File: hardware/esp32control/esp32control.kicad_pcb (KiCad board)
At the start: 2 copper layers, 67.6 x 85.9 mm, 76 parts, among them J1 Conn_02x10_Odd_Even, Q1 BSS138, Q2 BSS138, Q3 BSS138, Q4 BSS138, Q5 BSS138, Q6 BSS138, Q7 MMBT3904, Q8 MMBT3904, SW1 Boot, SW2 Reset, U1 ESP32-WROOM, U10 LTV-354T, U11 HUT4, U12 LM1117-3.3, U2 AQY212, U3 AQY212, U4 LM2675M-5, U5 LTV-354T, U6 AQY212, U7 AQY212, U8 LTV-354T, U9 LTV-354T

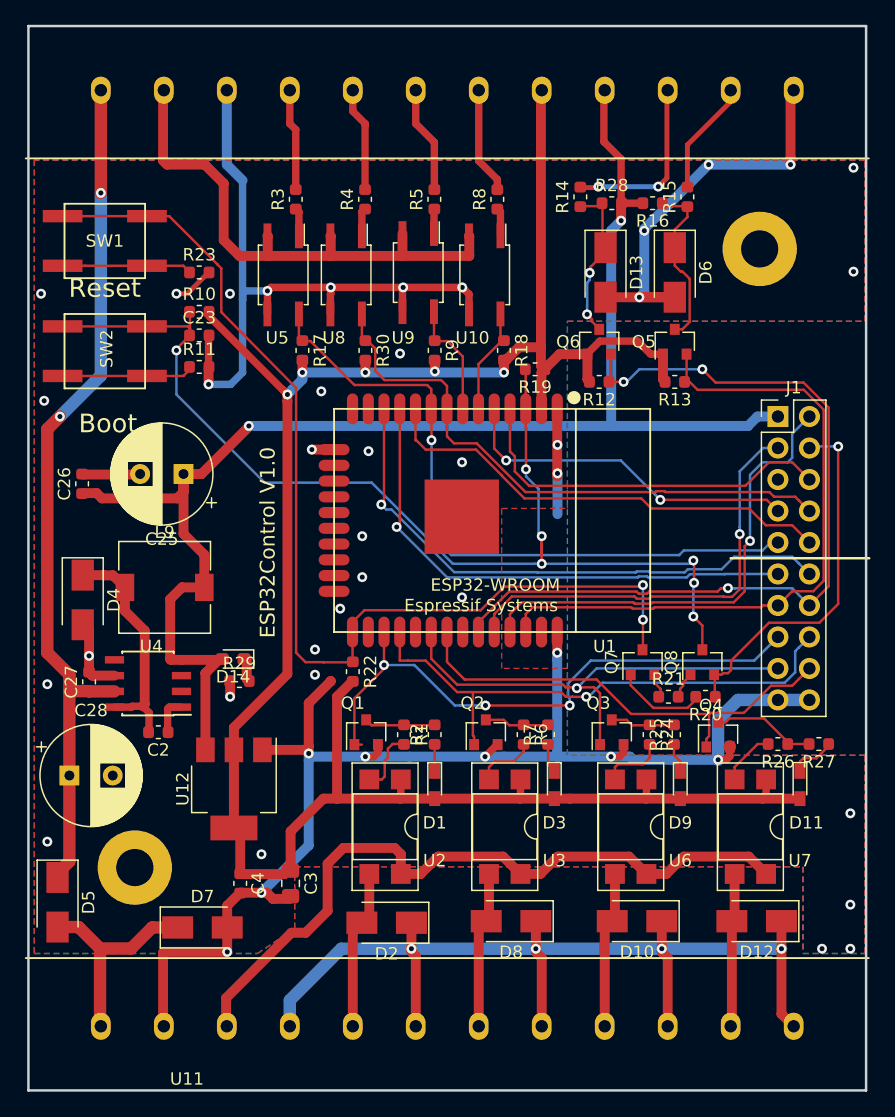
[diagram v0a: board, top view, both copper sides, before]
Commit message: silk update, fab files regen, pdf added
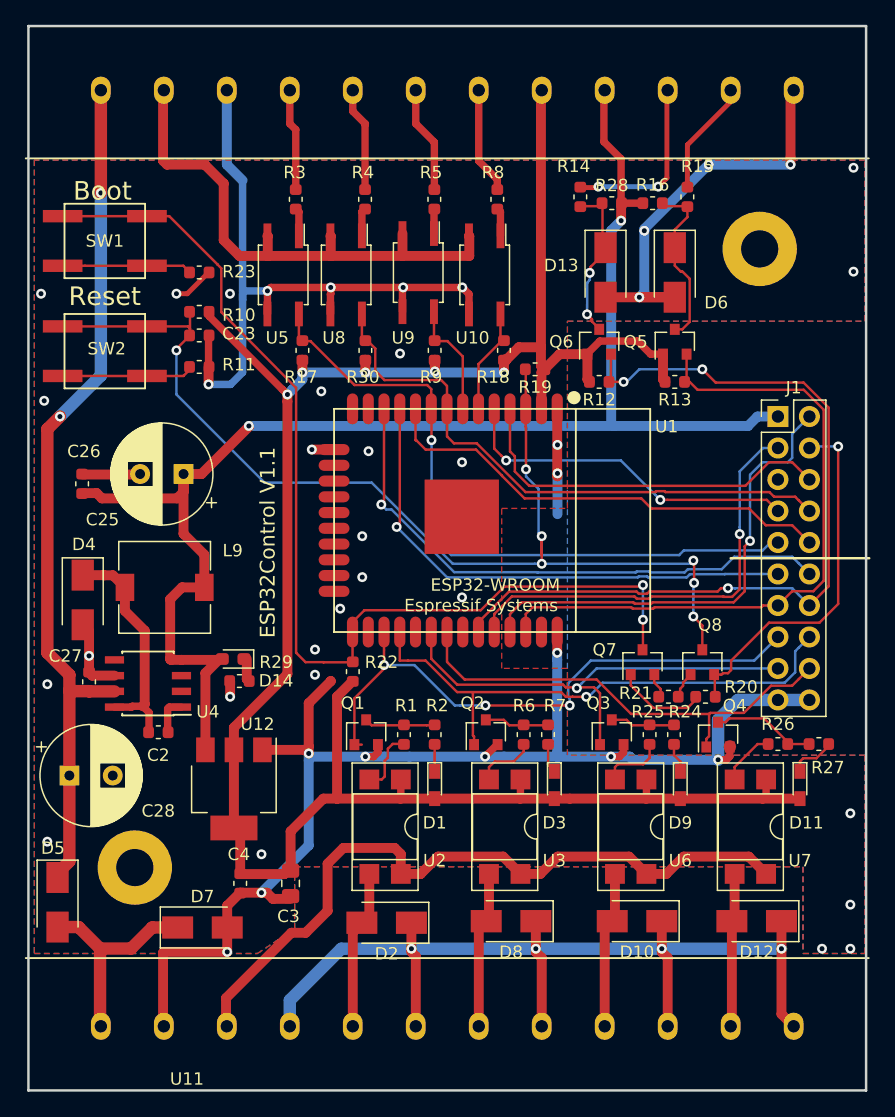
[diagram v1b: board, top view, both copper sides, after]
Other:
- board text added: "ESP32Control V1.1"
- board text removed: "ESP32Control V1.0"
